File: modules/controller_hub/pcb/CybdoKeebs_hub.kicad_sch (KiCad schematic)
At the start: 30 parts, among them SW1 BOOTSEL, SW2 RESET, U1 RP2350_60QFN, Y1 ABM8-272-T3

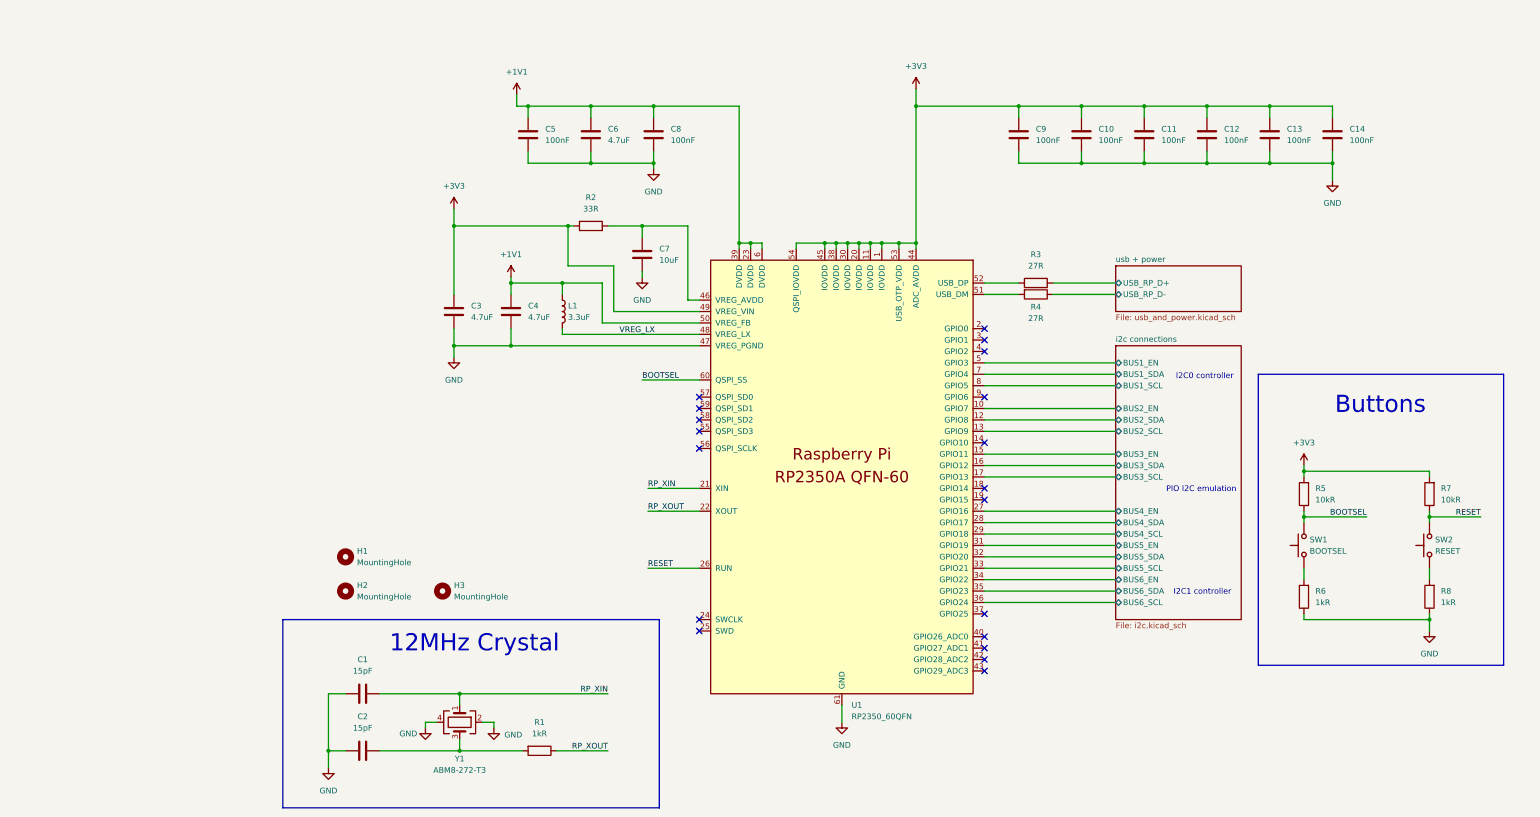
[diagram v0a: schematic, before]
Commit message: finished all pcbs
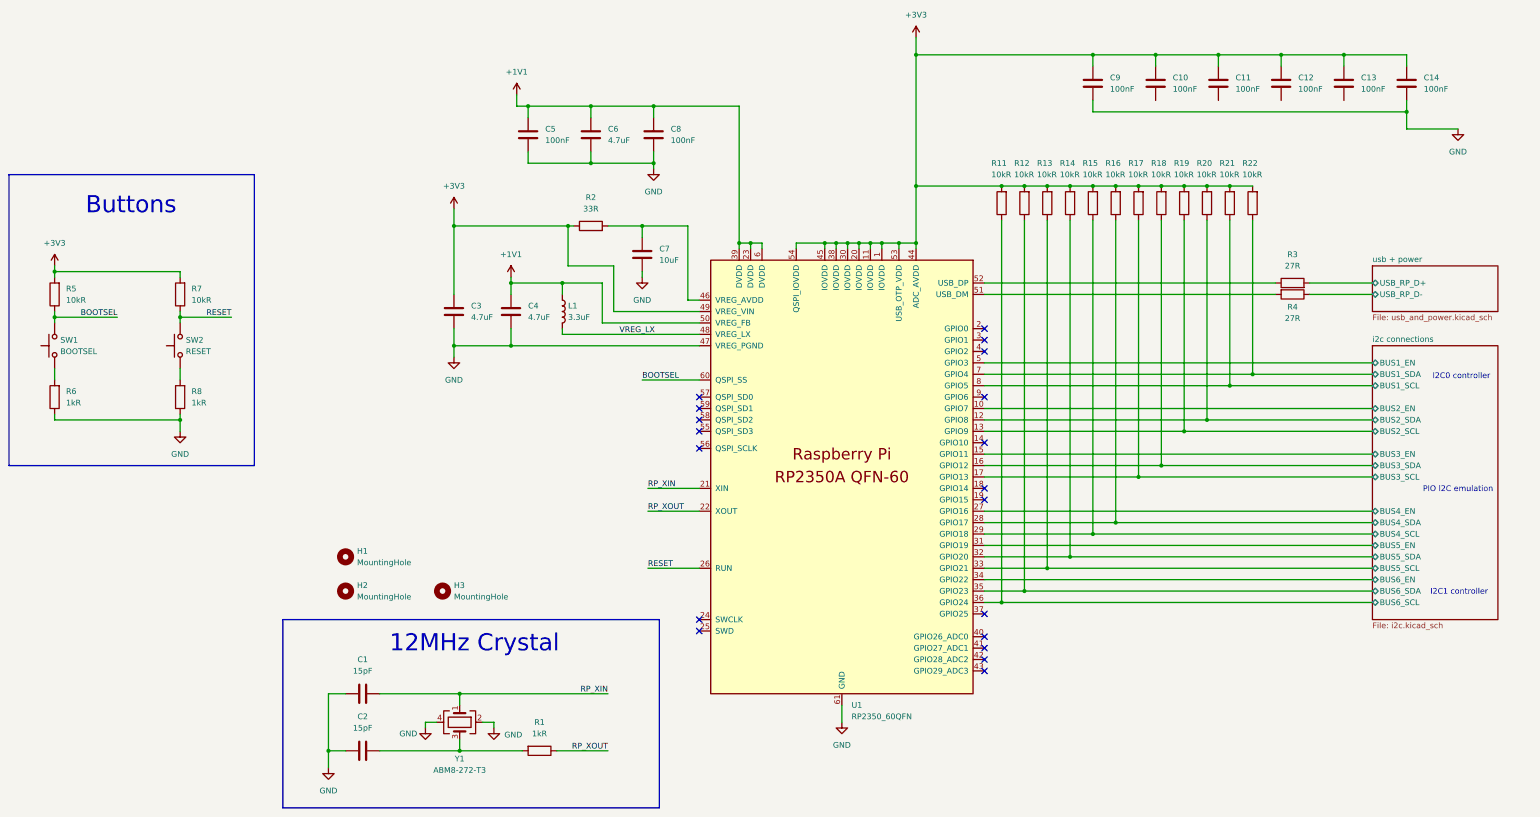
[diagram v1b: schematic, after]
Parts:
- added R11, R12, R13, R14, R15, R16, R17, R18, R19, R20, R21, R22: 10kR, Resistor_SMD:R_0402_1005Metric_Pad0.72x0.64mm_HandSolder, symbol Device:R
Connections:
- net +3V3: now also R11.2, R12.2, R13.2, R14.2, R15.2, R16.2, R17.2, R18.2, R19.2, R20.2, R21.2, R22.2
- net GND: no longer C10.2, C11.2, C12.2, C13.2
- net i2c connections/BUS1_SCL: now also R21.1
- net i2c connections/BUS1_SDA: now also R22.1
- net i2c connections/BUS2_SCL: now also R19.1
- net i2c connections/BUS2_SDA: now also R20.1
- net i2c connections/BUS3_SCL: now also R17.1
- net i2c connections/BUS3_SDA: now also R18.1
- net i2c connections/BUS4_SCL: now also R15.1
- net i2c connections/BUS4_SDA: now also R16.1
- net i2c connections/BUS5_SCL: now also R13.1
- net i2c connections/BUS5_SDA: now also R14.1
- net i2c connections/BUS6_SCL: now also R11.1
- net i2c connections/BUS6_SDA: now also R12.1
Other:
- moved on the sheet: C10, C11, C12, C13, C14, C9, R3, R4, R5, R6, R7, R8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
